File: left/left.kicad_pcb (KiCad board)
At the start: 2 copper layers, 51 parts, among them J1 MJ-4PP-9, U1 ProMicro

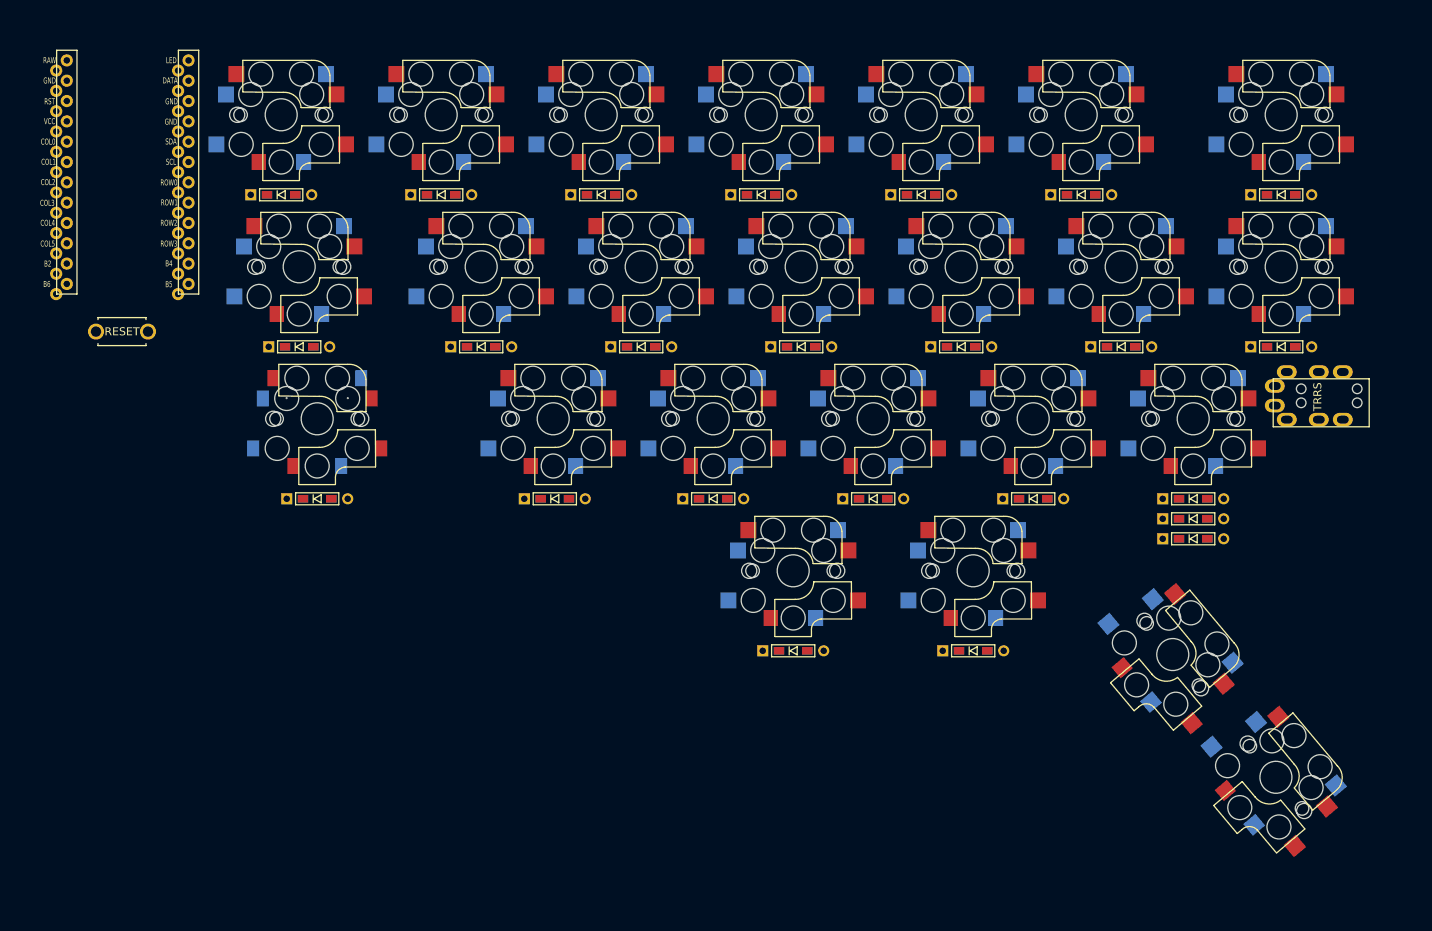
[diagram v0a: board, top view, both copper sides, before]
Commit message: 左手PCB完成
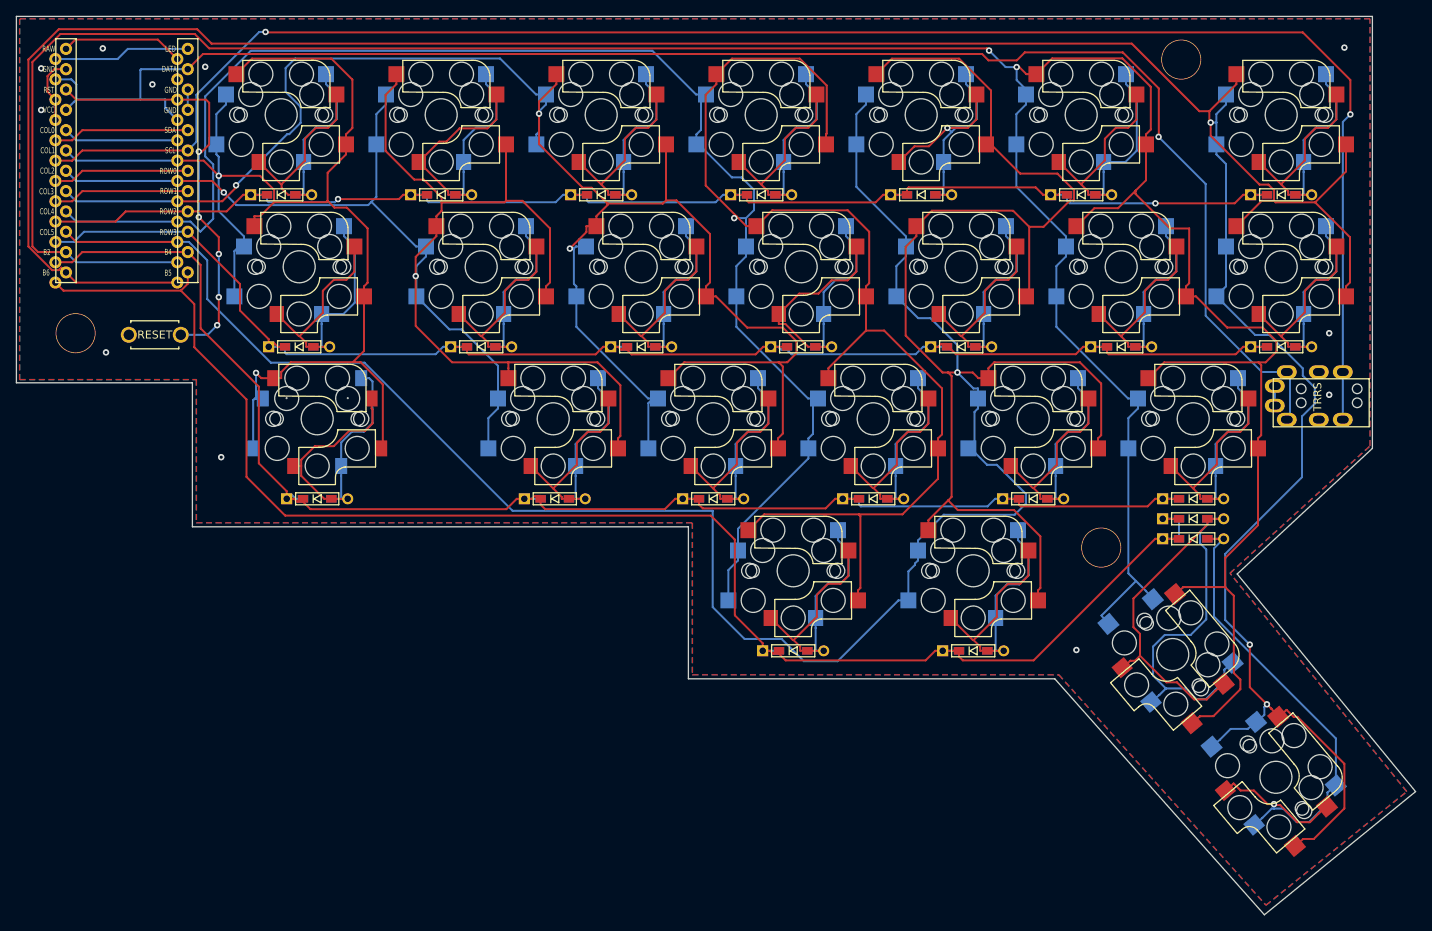
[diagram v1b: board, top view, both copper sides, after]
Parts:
- added Ref01: Val01, kbd:HOLE, F.Cu at (40.4, 74.8)
- added Ref02: Val02, kbd:HOLE, F.Cu at (178.6, 40.6)
- added Ref03: Val03, kbd:HOLE, F.Cu at (168.6, 101.6)
- moved LEFT_SW_RESET1 4.12 mm to (50.3, 75.0)
- moved U1 1.44 mm to (46.8, 53.7)
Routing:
- net col6: track 0.00 -> 403.2 mm, vias 0 -> 2
- net col5: track 0.00 -> 392.6 mm, vias 0 -> 1
- net col7: track 0.00 -> 380.7 mm, vias 0 -> 3
- net col4: track 0.00 -> 326.7 mm, vias 0 -> 1
- net col3: track 0.00 -> 218.7 mm, vias 0 -> 3
- net data: track 0.00 -> 217.3 mm, vias 0 -> 2
- net pwr: track 0.00 -> 205.5 mm, vias 0 -> 1
- net col2: track 0.00 -> 201.3 mm, vias 0 -> 2
- net row4: track 0.00 -> 198.3 mm
- net row3: track 0.00 -> 184.7 mm
- net row2: track 0.00 -> 182.1 mm
- net row1: track 0.00 -> 174.9 mm, vias 0 -> 2
- net col1: track 0.00 -> 163.0 mm, vias 0 -> 2
- net Net-(D23-A): track 0.00 -> 83.0 mm
- net Net-(D24-A): track 0.00 -> 72.4 mm, vias 0 -> 1
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- added copper zone on B.Cu, net GND
- added copper zone on F.Cu, net GND
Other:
- board outline added: 174.9 x 112.3 mm
